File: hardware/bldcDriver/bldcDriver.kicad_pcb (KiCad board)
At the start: 2 copper layers, 89.8 x 41.5 mm, 4 parts

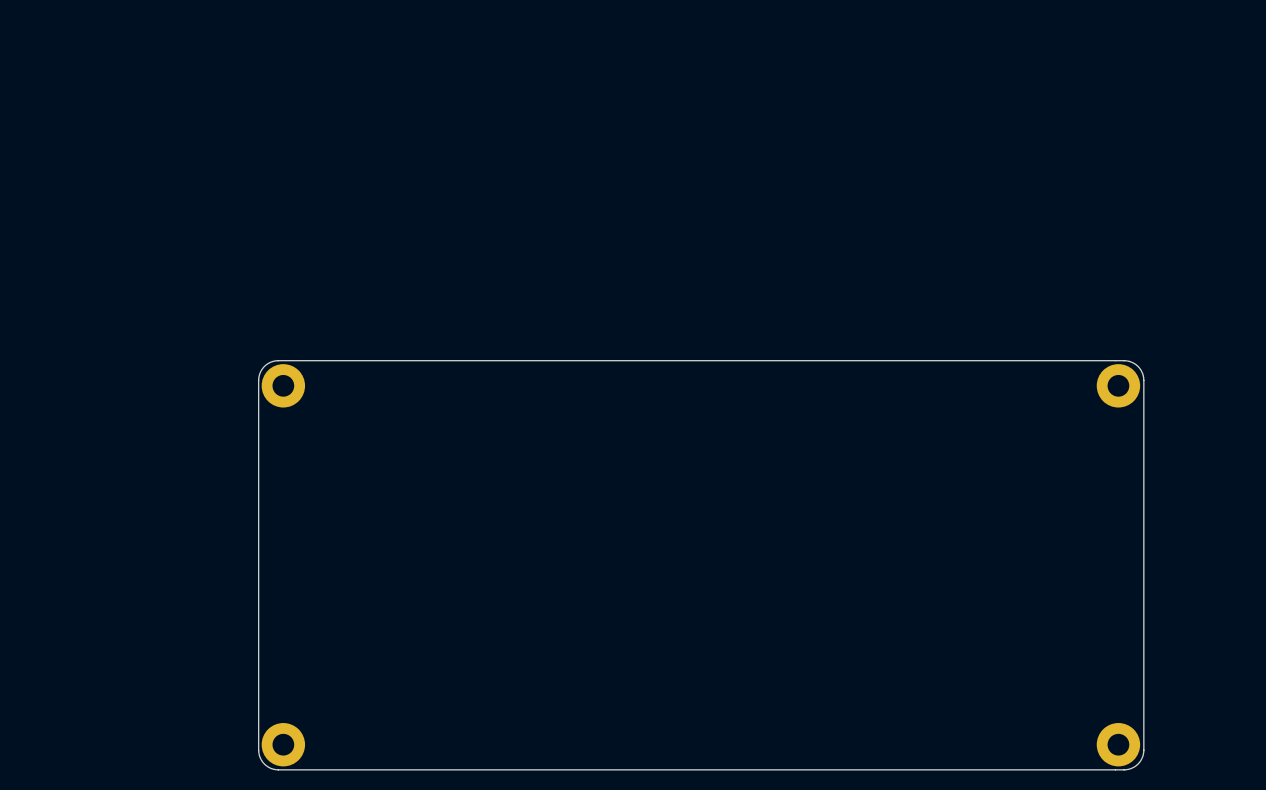
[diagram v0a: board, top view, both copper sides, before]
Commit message: update driver pcb
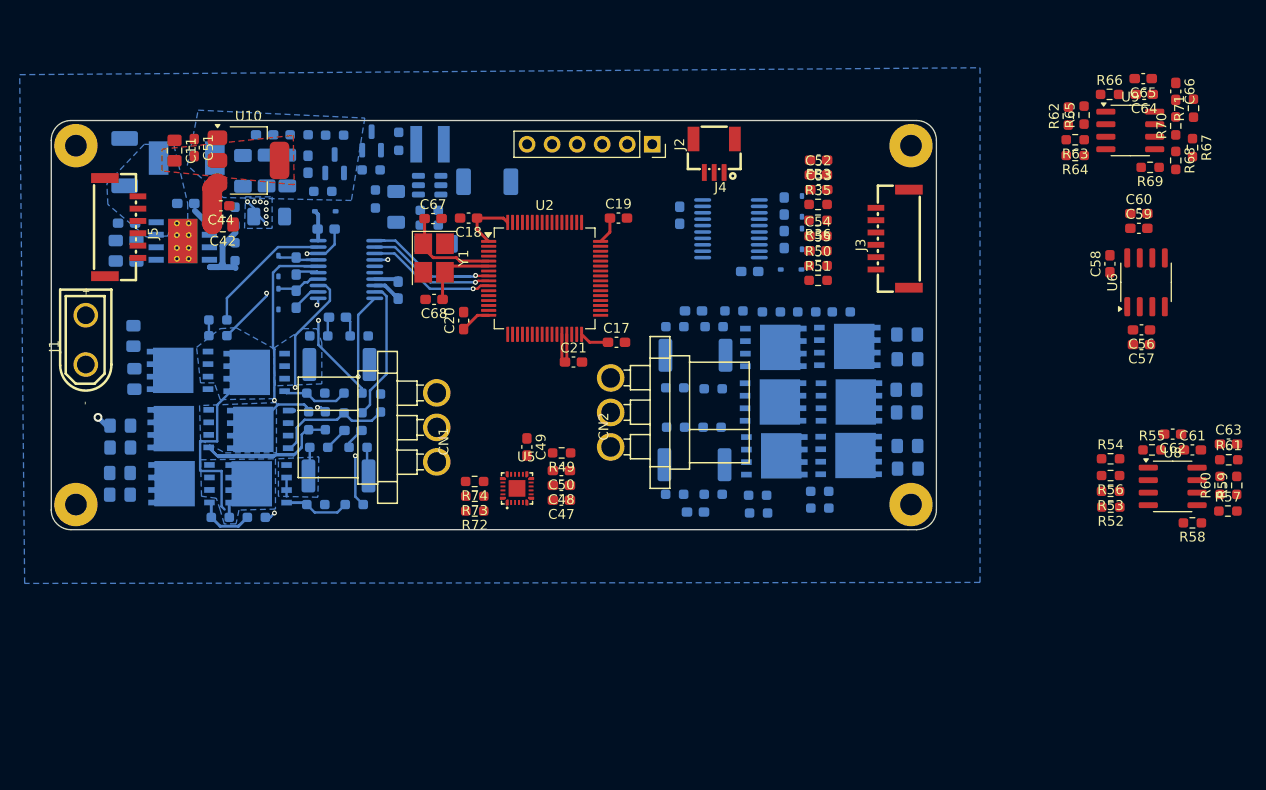
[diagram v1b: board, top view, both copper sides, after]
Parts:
- added C1: 10n, Capacitor_SMD:C_0603_1608Metric_Pad1.08x0.95mm_HandSolder, B.Cu at (46.1, 39.1)
- added C10: 47u, Capacitor_SMD:C_1206_3216Metric_Pad1.33x1.80mm_HandSolder, B.Cu at (71.5, 43.2)
- added C11: 10u, Capacitor_SMD:C_0805_2012Metric_Pad1.18x1.45mm_HandSolder, F.Cu at (45.0, 33.7)
- added C12: 100nF/25V, Capacitor_SMD:C_0603_1608Metric_Pad1.08x0.95mm_HandSolder, B.Cu at (96.2, 40.3)
- added C14: 100n, Capacitor_SMD:C_0603_1608Metric_Pad1.08x0.95mm_HandSolder, B.Cu at (103.3, 46.0)
- added C15: 100n, Capacitor_SMD:C_0603_1608Metric_Pad1.08x0.95mm_HandSolder, B.Cu at (106.8, 42.8)
- added C16: 100n, Capacitor_SMD:C_0603_1608Metric_Pad1.08x0.95mm_HandSolder, B.Cu at (106.8, 39.4)
- added C17: 100n, Capacitor_SMD:C_0603_1608Metric_Pad1.08x0.95mm_HandSolder, F.Cu at (89.8, 53.2)
- added C18: 100n, Capacitor_SMD:C_0603_1608Metric_Pad1.08x0.95mm_HandSolder, F.Cu at (74.8, 40.6)
- added C19: 100n, Capacitor_SMD:C_0603_1608Metric_Pad1.08x0.95mm_HandSolder, F.Cu at (90.0, 40.6)
- added C2: 47u, Capacitor_SMD:C_1206_3216Metric_Pad1.33x1.80mm_HandSolder, B.Cu at (56.4, 35.8)
- added C20: 100n, Capacitor_SMD:C_0603_1608Metric_Pad1.08x0.95mm_HandSolder, F.Cu at (74.3, 51.0)
- added C21: 470n, Capacitor_SMD:C_0603_1608Metric_Pad1.08x0.95mm_HandSolder, F.Cu at (85.4, 55.2)
- added C25: 100nF/25V, Capacitor_SMD:C_0603_1608Metric_Pad1.08x0.95mm_HandSolder, B.Cu at (67.6, 47.9)
- added C26: 100n, Capacitor_SMD:C_0603_1608Metric_Pad1.08x0.95mm_HandSolder, B.Cu at (60.3, 41.7)
- added C27: 100n, Capacitor_SMD:C_0603_1608Metric_Pad1.08x0.95mm_HandSolder, B.Cu at (57.3, 45.5)
- added C28: 100n, Capacitor_SMD:C_0603_1608Metric_Pad1.08x0.95mm_HandSolder, B.Cu at (57.3, 48.8)
- added C29: 22uF/25V, Capacitor_SMD:C_0805_2012Metric_Pad1.18x1.45mm_HandSolder, B.Cu at (40.8, 52.5)
- added C3: 47u, Capacitor_SMD:C_1206_3216Metric_Pad1.33x1.80mm_HandSolder, B.Cu at (54.3, 35.8)
- added C30: 1n, Capacitor_SMD:C_0603_1608Metric_Pad1.08x0.95mm_HandSolder, B.Cu at (61.5, 50.6)
- added C31: 22uF/25V, Capacitor_SMD:C_0805_2012Metric_Pad1.18x1.45mm_HandSolder, B.Cu at (119.3, 52.4)
- added C32: 1n, Capacitor_SMD:C_0603_1608Metric_Pad1.08x0.95mm_HandSolder, B.Cu at (97.6, 50.0)
- added C33: 22uF/25V, Capacitor_SMD:C_0805_2012Metric_Pad1.18x1.45mm_HandSolder, B.Cu at (40.9, 56.9)
- added C34: 22uF/25V, Capacitor_SMD:C_0805_2012Metric_Pad1.18x1.45mm_HandSolder, B.Cu at (119.3, 54.9)
- added C35: 22uF/25V, Capacitor_SMD:C_0805_2012Metric_Pad1.18x1.45mm_HandSolder, B.Cu at (39.4, 66.4)
- added C36: 1n, Capacitor_SMD:C_0603_1608Metric_Pad1.08x0.95mm_HandSolder, B.Cu at (63.1, 62.1)
- added C37: 22uF/25V, Capacitor_SMD:C_0805_2012Metric_Pad1.18x1.45mm_HandSolder, B.Cu at (119.3, 66.0)
- added C38: 1n, Capacitor_SMD:C_0603_1608Metric_Pad1.08x0.95mm_HandSolder, B.Cu at (97.8, 70.4)
- added C39: 22uF/25V, Capacitor_SMD:C_0805_2012Metric_Pad1.18x1.45mm_HandSolder, B.Cu at (39.4, 68.6)
- added C4: 47u, Capacitor_SMD:C_1206_3216Metric_Pad1.33x1.80mm_HandSolder, B.Cu at (51.9, 35.8)
- added C40: 22uF/25V, Capacitor_SMD:C_0805_2012Metric_Pad1.18x1.45mm_HandSolder, B.Cu at (119.3, 63.7)
- added C41: 22uF/25V, Capacitor_SMD:C_0805_2012Metric_Pad1.18x1.45mm_HandSolder, B.Cu at (39.5, 61.6)
- added C42: 10u, Capacitor_SMD:C_0805_2012Metric_Pad1.18x1.45mm_HandSolder, F.Cu at (49.9, 41.2)
- added C43: 22uF/25V, Capacitor_SMD:C_0805_2012Metric_Pad1.18x1.45mm_HandSolder, B.Cu at (119.2, 58.0)
- added C44: 100n, Capacitor_SMD:C_0603_1608Metric_Pad1.08x0.95mm_HandSolder, F.Cu at (49.7, 39.3)
- added C45: 22uF/25V, Capacitor_SMD:C_0805_2012Metric_Pad1.18x1.45mm_HandSolder, B.Cu at (39.5, 63.9)
- added C46: 22uF/25V, Capacitor_SMD:C_0805_2012Metric_Pad1.18x1.45mm_HandSolder, B.Cu at (119.2, 60.3)
- added C47: 10n, Capacitor_SMD:C_0603_1608Metric_Pad1.08x0.95mm_HandSolder, F.Cu at (84.2, 69.2)
- added C48: 100n, Capacitor_SMD:C_0603_1608Metric_Pad1.08x0.95mm_HandSolder, F.Cu at (84.2, 67.7)
- added C49: 2.2U, Capacitor_SMD:C_0603_1608Metric_Pad1.08x0.95mm_HandSolder, F.Cu at (80.7, 63.8)
- added C5: 22u, Capacitor_SMD:C_0805_2012Metric_Pad1.18x1.45mm_HandSolder, B.Cu at (39.0, 43.9)
- added C50: 100n, Capacitor_SMD:C_0603_1608Metric_Pad1.08x0.95mm_HandSolder, F.Cu at (84.2, 66.2)
- added C51: 100n, Capacitor_SMD:C_0603_1608Metric_Pad1.08x0.95mm_HandSolder, F.Cu at (47.0, 33.4)
- added C52: 4.7u, Capacitor_SMD:C_0603_1608Metric_Pad1.08x0.95mm_HandSolder, F.Cu at (110.3, 36.2)
- added C53: 100n, Capacitor_SMD:C_0603_1608Metric_Pad1.08x0.95mm_HandSolder, F.Cu at (110.3, 37.7)
- added C54: 4.7u, Capacitor_SMD:C_0603_1608Metric_Pad1.08x0.95mm_HandSolder, F.Cu at (110.2, 42.4)
- added C55: 100n, Capacitor_SMD:C_0603_1608Metric_Pad1.08x0.95mm_HandSolder, F.Cu at (110.2, 43.9)
- added C56: 4.7u, Capacitor_SMD:C_0603_1608Metric_Pad1.08x0.95mm_HandSolder, F.Cu at (143.0, 51.9)
- added C57: 100n, Capacitor_SMD:C_0603_1608Metric_Pad1.08x0.95mm_HandSolder, F.Cu at (143.0, 53.4)
- added C58: 100n, Capacitor_SMD:C_0603_1608Metric_Pad1.08x0.95mm_HandSolder, F.Cu at (139.8, 45.2)
- added C59: 4.7u, Capacitor_SMD:C_0603_1608Metric_Pad1.08x0.95mm_HandSolder, F.Cu at (142.8, 41.6)
- added C6: 22u, Capacitor_SMD:C_0805_2012Metric_Pad1.18x1.45mm_HandSolder, B.Cu at (41.1, 43.9)
- added C60: 100n, Capacitor_SMD:C_0603_1608Metric_Pad1.08x0.95mm_HandSolder, F.Cu at (142.8, 40.1)
- added C61: 100n, Capacitor_SMD:C_0603_1608Metric_Pad1.08x0.95mm_HandSolder, F.Cu at (148.2, 64.1)
- added C62: 2.2n, Capacitor_SMD:C_0603_1608Metric_Pad1.08x0.95mm_HandSolder, F.Cu at (146.2, 62.5)
- added C63: 2.2n, Capacitor_SMD:C_0603_1608Metric_Pad1.08x0.95mm_HandSolder, F.Cu at (151.9, 63.5)
- added C64: 2.2n, Capacitor_SMD:C_0603_1608Metric_Pad1.08x0.95mm_HandSolder, F.Cu at (143.3, 28.0)
- added C65: 2.2n, Capacitor_SMD:C_0603_1608Metric_Pad1.08x0.95mm_HandSolder, F.Cu at (143.2, 26.4)
- added C66: 100n, Capacitor_SMD:C_0603_1608Metric_Pad1.08x0.95mm_HandSolder, F.Cu at (146.5, 27.7)
- added C67: 12p, Capacitor_SMD:C_0603_1608Metric_Pad1.08x0.95mm_HandSolder, F.Cu at (71.2, 40.6)
- added C68: 12p, Capacitor_SMD:C_0603_1608Metric_Pad1.08x0.95mm_HandSolder, F.Cu at (71.3, 48.8)
- added C7: 100n, Capacitor_SMD:C_0603_1608Metric_Pad1.08x0.95mm_HandSolder, B.Cu at (40.1, 41.1)
- added C8: 100n, Capacitor_SMD:C_0603_1608Metric_Pad1.08x0.95mm_HandSolder, B.Cu at (58.5, 35.1)
- added C9: 47u, Capacitor_SMD:C_1206_3216Metric_Pad1.33x1.80mm_HandSolder, B.Cu at (67.4, 39.5)
- added CN1: MR30PW-F, balancerDriver:CONN-TH_MR30PW-F, F.Cu at (69.1, 61.8)
- added CN2: MR30PW-F, balancerDriver:CONN-TH_MR30PW-F, F.Cu at (91.7, 60.3)
- added D1: LED, LED_SMD:LED_0603_1608Metric_Pad1.05x0.95mm_HandSolder, B.Cu at (54.1, 32.1)
- added D10: 1N5819WS, Diode_SMD:D_SOD-323, B.Cu at (60.2, 39.9)
- added D11: 1N5819WS, Diode_SMD:D_SOD-323, B.Cu at (55.5, 45.5)
- added D12: 1N5819WS, Diode_SMD:D_SOD-323, B.Cu at (55.5, 48.8)
- added D2: 1N5819WS, Diode_SMD:D_SOD-323, B.Cu at (107.5, 45.8)
- added D3: 1N5819WS, Diode_SMD:D_SOD-323, B.Cu at (108.6, 42.7)
- added D4: 1N5819WS, Diode_SMD:D_SOD-323, B.Cu at (108.6, 39.4)
- added D8: 1N5712UR, Diode_SMD:D_MELF, B.Cu at (39.9, 34.9)
- added D9: 1N5712UR, Diode_SMD:D_MELF, B.Cu at (76.7, 36.9)
- added FB2: FerriteBead, Capacitor_SMD:C_1206_3216Metric_Pad1.33x1.80mm_HandSolder, B.Cu at (54.6, 40.4)
- added FB3: FerriteBead, Capacitor_SMD:C_0603_1608Metric_Pad1.08x0.95mm_HandSolder, F.Cu at (110.3, 34.7)
- added J1: Conn_01x02, balancerDriver:CONN-TH_XT30UPB-M, F.Cu at (36.0, 52.9)
- added J2: Conn_01x06, Connector_PinSocket_2.54mm:PinSocket_1x06_P2.54mm_Vertical, F.Cu at (93.4, 33.1)
- added J3: Conn_01x06, balancerDriver:CONN-SMD_BM06B-GHS-TBT-LF-SN, F.Cu at (117.8, 42.7)
- added J4: Conn_01x03, balancerDriver:CONN-SMD_3P-P1.00_WAFER-SH1.0-3PWB, F.Cu at (99.7, 34.3)
- added J5: Conn_01x06, balancerDriver:CONN-SMD_BM06B-GHS-TBT-LF-SN, F.Cu at (39.6, 41.5)
- added L1: 10u, Inductor_SMD:L_Sumida_CDMC6D28_7.25x6.5mm, B.Cu at (46.2, 34.5)
- added L2: 10u, Inductor_SMD:L_Taiyo-Yuden_MD-4040, B.Cu at (70.9, 33.1)
- added Q1: KNY3406C, balancerDriver:PDFN-8_L4.9-W5.8-P1.27-LS6.1-BL, B.Cu at (45.5, 56.0)
- added Q10: KNY3406C, balancerDriver:PDFN-8_L4.9-W5.8-P1.27-LS6.1-BL, B.Cu at (53.7, 62.0)
- added Q11: KNY3406C, balancerDriver:PDFN-8_L4.9-W5.8-P1.27-LS6.1-BL, B.Cu at (113.4, 59.2)
- added Q12: KNY3406C, balancerDriver:PDFN-8_L4.9-W5.8-P1.27-LS6.1-BL, B.Cu at (105.7, 59.2)
- added Q13: PMOS, Package_TO_SOT_SMD:SOT-23, B.Cu at (61.2, 35.1)
- added Q14: S8050, Package_TO_SOT_SMD:SOT-23, B.Cu at (65.0, 32.8)
- added Q2: KNY3406C, balancerDriver:PDFN-8_L4.9-W5.8-P1.27-LS6.1-BL, B.Cu at (53.3, 56.2)
- added Q3: KNY3406C, balancerDriver:PDFN-8_L4.9-W5.8-P1.27-LS6.1-BL, B.Cu at (113.2, 53.6)
- added Q4: KNY3406C, balancerDriver:PDFN-8_L4.9-W5.8-P1.27-LS6.1-BL, B.Cu at (105.7, 53.7)
- added Q5: KNY3406C, balancerDriver:PDFN-8_L4.9-W5.8-P1.27-LS6.1-BL, B.Cu at (45.7, 67.5)
- added Q6: KNY3406C, balancerDriver:PDFN-8_L4.9-W5.8-P1.27-LS6.1-BL, B.Cu at (53.5, 67.5)
- added Q7: KNY3406C, balancerDriver:PDFN-8_L4.9-W5.8-P1.27-LS6.1-BL, B.Cu at (113.3, 64.7)
- added Q8: KNY3406C, balancerDriver:PDFN-8_L4.9-W5.8-P1.27-LS6.1-BL, B.Cu at (105.8, 64.7)
- added Q9: KNY3406C, balancerDriver:PDFN-8_L4.9-W5.8-P1.27-LS6.1-BL, B.Cu at (45.6, 61.9)
- added R1: 10k, Resistor_SMD:R_0603_1608Metric_Pad0.98x0.95mm_HandSolder, B.Cu at (51.1, 40.4)
- added R10: 100R, Resistor_SMD:R_0603_1608Metric_Pad0.98x0.95mm_HandSolder, B.Cu at (95.7, 51.6)
- added R11: 20mR, Resistor_SMD:R_2512_6332Metric_Pad1.40x3.35mm_HandSolder, B.Cu at (61.7, 55.4)
- added R12: 20mR, Resistor_SMD:R_2512_6332Metric_Pad1.40x3.35mm_HandSolder, B.Cu at (97.8, 54.5)
- added R13: 10k, Resistor_SMD:R_0603_1608Metric_Pad0.98x0.95mm_HandSolder, B.Cu at (49.4, 52.5)
- added R14: 10k, Resistor_SMD:R_0603_1608Metric_Pad0.98x0.95mm_HandSolder, B.Cu at (59.3, 58.3)
- added R15: 10k, Resistor_SMD:R_0603_1608Metric_Pad0.98x0.95mm_HandSolder, B.Cu at (112.6, 50.1)
- added R16: 10k, Resistor_SMD:R_0603_1608Metric_Pad0.98x0.95mm_HandSolder, B.Cu at (105.5, 50.1)
- added R17: 10R, Resistor_SMD:R_0603_1608Metric_Pad0.98x0.95mm_HandSolder, B.Cu at (49.4, 50.9)
- added R18: 10R, Resistor_SMD:R_0603_1608Metric_Pad0.98x0.95mm_HandSolder, B.Cu at (63.1, 58.3)
- added R19: 10R, Resistor_SMD:R_0603_1608Metric_Pad0.98x0.95mm_HandSolder, B.Cu at (109.1, 50.1)
- added R2: 3.3k, Resistor_SMD:R_0603_1608Metric_Pad0.98x0.95mm_HandSolder, B.Cu at (51.1, 44.0)
- added R20: 10R, Resistor_SMD:R_0603_1608Metric_Pad0.98x0.95mm_HandSolder, B.Cu at (101.7, 50.0)
- added R21: 100R, Resistor_SMD:R_0603_1608Metric_Pad0.98x0.95mm_HandSolder, B.Cu at (59.6, 63.8)
- added R22: 100R, Resistor_SMD:R_0603_1608Metric_Pad0.98x0.95mm_HandSolder, B.Cu at (63.6, 63.8)
- added R23: 100R, Resistor_SMD:R_0603_1608Metric_Pad0.98x0.95mm_HandSolder, B.Cu at (99.6, 68.6)
- added R24: 100R, Resistor_SMD:R_0603_1608Metric_Pad0.98x0.95mm_HandSolder, B.Cu at (95.7, 68.6)
- added R25: 20mR, Resistor_SMD:R_2512_6332Metric_Pad1.40x3.35mm_HandSolder, B.Cu at (61.6, 66.7)
- added R26: 20mR, Resistor_SMD:R_2512_6332Metric_Pad1.40x3.35mm_HandSolder, B.Cu at (97.7, 65.6)
- added R27: 10k, Resistor_SMD:R_0603_1608Metric_Pad0.98x0.95mm_HandSolder, B.Cu at (49.6, 70.9)
- added R28: 10k, Resistor_SMD:R_0603_1608Metric_Pad0.98x0.95mm_HandSolder, B.Cu at (59.3, 69.6)
- added R29: 10k, Resistor_SMD:R_0603_1608Metric_Pad0.98x0.95mm_HandSolder, B.Cu at (110.4, 68.3)
- added R3: 4.7k, Resistor_SMD:R_0603_1608Metric_Pad0.98x0.95mm_HandSolder, B.Cu at (57.6, 32.1)
- added R30: 10k, Resistor_SMD:R_0603_1608Metric_Pad0.98x0.95mm_HandSolder, B.Cu at (104.1, 68.7)
- added R31: 10R, Resistor_SMD:R_0603_1608Metric_Pad0.98x0.95mm_HandSolder, B.Cu at (53.3, 70.9)
- added R32: 10R, Resistor_SMD:R_0603_1608Metric_Pad0.98x0.95mm_HandSolder, B.Cu at (63.2, 69.6)
- added R33: 10R, Resistor_SMD:R_0603_1608Metric_Pad0.98x0.95mm_HandSolder, B.Cu at (110.4, 70.0)
- added R34: 10R, Resistor_SMD:R_0603_1608Metric_Pad0.98x0.95mm_HandSolder, B.Cu at (104.2, 70.5)
- added R35: 1k, Resistor_SMD:R_0603_1608Metric_Pad0.98x0.95mm_HandSolder, F.Cu at (110.2, 39.2)
- added R36: 1k, Resistor_SMD:R_0603_1608Metric_Pad0.98x0.95mm_HandSolder, F.Cu at (110.2, 40.8)
- added R37: 10k, Resistor_SMD:R_0603_1608Metric_Pad0.98x0.95mm_HandSolder, B.Cu at (64.9, 35.7)
- added R38: 10k, Resistor_SMD:R_0603_1608Metric_Pad0.98x0.95mm_HandSolder, B.Cu at (65.3, 38.6)
- added R39: 63.4k, Resistor_SMD:R_0603_1608Metric_Pad0.98x0.95mm_HandSolder, B.Cu at (70.8, 41.3)
- added R4: 10k, Resistor_SMD:R_0603_1608Metric_Pad0.98x0.95mm_HandSolder, B.Cu at (60.0, 37.9)
- added R40: 3.3k, Resistor_SMD:R_0603_1608Metric_Pad0.98x0.95mm_HandSolder, B.Cu at (70.8, 39.8)
- added R41: 10k, Resistor_SMD:R_0603_1608Metric_Pad0.98x0.95mm_HandSolder, B.Cu at (58.6, 61.1)
- added R42: 10k, Resistor_SMD:R_0603_1608Metric_Pad0.98x0.95mm_HandSolder, B.Cu at (65.9, 59.3)
- added R43: 10k, Resistor_SMD:R_0603_1608Metric_Pad0.98x0.95mm_HandSolder, B.Cu at (99.5, 61.8)
- added R44: 10k, Resistor_SMD:R_0603_1608Metric_Pad0.98x0.95mm_HandSolder, B.Cu at (99.6, 57.9)
- added R45: 10R, Resistor_SMD:R_0603_1608Metric_Pad0.98x0.95mm_HandSolder, B.Cu at (60.3, 61.1)
- added R46: 10R, Resistor_SMD:R_0603_1608Metric_Pad0.98x0.95mm_HandSolder, B.Cu at (63.1, 60.3)
- added R47: 10R, Resistor_SMD:R_0603_1608Metric_Pad0.98x0.95mm_HandSolder, B.Cu at (95.8, 61.8)
- added R48: 10R, Resistor_SMD:R_0603_1608Metric_Pad0.98x0.95mm_HandSolder, B.Cu at (95.7, 57.8)
- added R49: 10K, Resistor_SMD:R_0603_1608Metric_Pad0.98x0.95mm_HandSolder, F.Cu at (84.2, 64.4)
- added R5: 100R, Resistor_SMD:R_0603_1608Metric_Pad0.98x0.95mm_HandSolder, B.Cu at (61.2, 32.2)
- added R50: 1k, Resistor_SMD:R_0603_1608Metric_Pad0.98x0.95mm_HandSolder, F.Cu at (110.2, 45.4)
- added R51: 1k, Resistor_SMD:R_0603_1608Metric_Pad0.98x0.95mm_HandSolder, F.Cu at (110.2, 46.9)
- added R52: 10k, Resistor_SMD:R_0603_1608Metric_Pad0.98x0.95mm_HandSolder, F.Cu at (139.9, 69.9)
- added R53: 1k, Resistor_SMD:R_0603_1608Metric_Pad0.98x0.95mm_HandSolder, F.Cu at (139.9, 68.3)
- added R54: 10k, Resistor_SMD:R_0603_1608Metric_Pad0.98x0.95mm_HandSolder, F.Cu at (139.9, 65.0)
- added R55: 100R, Resistor_SMD:R_0603_1608Metric_Pad0.98x0.95mm_HandSolder, F.Cu at (144.1, 64.1)
- added R56: 1k, Resistor_SMD:R_0603_1608Metric_Pad0.98x0.95mm_HandSolder, F.Cu at (139.9, 66.7)
- added R57: 1k, Resistor_SMD:R_0603_1608Metric_Pad0.98x0.95mm_HandSolder, F.Cu at (151.8, 70.3)
- added R58: 10k, Resistor_SMD:R_0603_1608Metric_Pad0.98x0.95mm_HandSolder, F.Cu at (148.2, 71.5)
- added R59: 1k, Resistor_SMD:R_0603_1608Metric_Pad0.98x0.95mm_HandSolder, F.Cu at (152.7, 67.7)
- added R6: 1k, Resistor_SMD:R_0603_1608Metric_Pad0.98x0.95mm_HandSolder, B.Cu at (67.7, 32.8)
- added R60: 10k, Resistor_SMD:R_0603_1608Metric_Pad0.98x0.95mm_HandSolder, F.Cu at (151.0, 67.7)
- added R61: 100R, Resistor_SMD:R_0603_1608Metric_Pad0.98x0.95mm_HandSolder, F.Cu at (151.9, 65.1)
- added R62: 1k, Resistor_SMD:R_0603_1608Metric_Pad0.98x0.95mm_HandSolder, F.Cu at (135.6, 30.2)
- added R63: 1k, Resistor_SMD:R_0603_1608Metric_Pad0.98x0.95mm_HandSolder, F.Cu at (136.3, 32.6)
- added R64: 10k, Resistor_SMD:R_0603_1608Metric_Pad0.98x0.95mm_HandSolder, F.Cu at (136.3, 34.2)
- added R65: 10k, Resistor_SMD:R_0603_1608Metric_Pad0.98x0.95mm_HandSolder, F.Cu at (137.2, 30.1)
- added R66: 100R, Resistor_SMD:R_0603_1608Metric_Pad0.98x0.95mm_HandSolder, F.Cu at (139.8, 28.0)
- added R67: 1k, Resistor_SMD:R_0603_1608Metric_Pad0.98x0.95mm_HandSolder, F.Cu at (148.2, 33.4)
- added R68: 1k, Resistor_SMD:R_0603_1608Metric_Pad0.98x0.95mm_HandSolder, F.Cu at (146.5, 34.7)
- added R69: 10k, Resistor_SMD:R_0603_1608Metric_Pad0.98x0.95mm_HandSolder, F.Cu at (143.9, 35.4)
- added R7: 100R, Resistor_SMD:R_0603_1608Metric_Pad0.98x0.95mm_HandSolder, B.Cu at (59.6, 52.5)
- added R70: 10k, Resistor_SMD:R_0603_1608Metric_Pad0.98x0.95mm_HandSolder, F.Cu at (146.5, 31.2)
- added R71: 100R, Resistor_SMD:R_0603_1608Metric_Pad0.98x0.95mm_HandSolder, F.Cu at (148.3, 29.4)
- added R72: 4.7k, Resistor_SMD:R_0603_1608Metric_Pad0.98x0.95mm_HandSolder, F.Cu at (75.4, 70.3)
- added R73: 4.7k, Resistor_SMD:R_0603_1608Metric_Pad0.98x0.95mm_HandSolder, F.Cu at (75.4, 68.8)
- added R74: 4.7k, Resistor_SMD:R_0603_1608Metric_Pad0.98x0.95mm_HandSolder, F.Cu at (75.4, 67.3)
- added R8: 100R, Resistor_SMD:R_0603_1608Metric_Pad0.98x0.95mm_HandSolder, B.Cu at (63.7, 52.5)
- added R9: 100R, Resistor_SMD:R_0603_1608Metric_Pad0.98x0.95mm_HandSolder, B.Cu at (99.7, 51.6)
- added U1: FD6288T, balancerDriver:TSSOP-20_L6.5-W4.4-P0.65-LS6.4-BL, B.Cu at (101.4, 41.7)
- added U10: AMS1117, Package_TO_SOT_SMD:SOT-223-3_TabPin2, F.Cu at (52.5, 34.7)
- added U11: FD6288T, balancerDriver:TSSOP-20_L6.5-W4.4-P0.65-LS6.4-BL, B.Cu at (62.4, 45.8)
- added U2: STM32G431RBTx, Package_QFP:LQFP-64_10x10mm_P0.5mm, F.Cu at (82.5, 46.7)
- added U3: TPS5430DDA, Package_SO:TI_SO-PowerPAD-8_ThermalVias, B.Cu at (45.8, 42.9)
- added U5: MPU6500, balancerDriver:QFN-24_L3.0-W3.0-P0.40-BL-EP, F.Cu at (79.7, 68.0)
- added U6: TLV9062xD, Package_SO:SOIC-8_3.9x4.9mm_P1.27mm, F.Cu at (143.5, 47.1)
- added U7: MT3608, Package_TO_SOT_SMD:SOT-23-6, B.Cu at (70.8, 37.2)
- added U8: TLV9062xD, Package_SO:SOIC-8_3.9x4.9mm_P1.27mm, F.Cu at (146.2, 67.8)
- added U9: TLV9062xD, Package_SO:SOIC-8_3.9x4.9mm_P1.27mm, F.Cu at (141.9, 31.7)
- added Y1: 25MHz, Crystal:Crystal_SMD_SeikoEpson_FA238-4Pin_3.2x2.5mm_HandSoldering, F.Cu at (71.3, 44.6)
- moved ? 32.2 mm to (35.0, 33.2)
- moved ? 32.2 mm to (35.0, 69.6)
- moved ? 32.2 mm to (119.7, 33.2)
- moved ? 32.2 mm to (119.7, 69.6)
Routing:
- net /inverter/1SH_U: track 0.00 -> 35.7 mm, vias 0 -> 2
- net /inverter/1GH_B: track 0.00 -> 31.8 mm, vias 0 -> 2
- net Net-(Q9-G): track 0.00 -> 24.0 mm
- net /inverter/1GL_B: track 0.00 -> 22.1 mm, vias 0 -> 2
- net +3V3: track 0.00 -> 20.8 mm
- net /inverter/1GH_C: track 0.00 -> 16.8 mm, vias 0 -> 2
- net /TIM1_CH1: track 0.00 -> 16.5 mm, vias 0 -> 1
- net /inverter/1GL_C: track 0.00 -> 14.2 mm
- net /inverter/1GH_A: track 0.00 -> 13.6 mm
- net /TIM1_CH3: track 0.00 -> 13.2 mm, vias 0 -> 1
- net /TIM1_CH2: track 0.00 -> 13.1 mm, vias 0 -> 1
- net Net-(Q10-G): track 0.00 -> 12.4 mm
- net /inverter/1GL_A: track 0.00 -> 11.6 mm, vias 0 -> 2
- net /YI: track 0.00 -> 10.2 mm
- net /inverter/1SH_V: track 0.00 -> 9.31 mm
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- added copper zone on F.Cu, net +3V3
- added copper zone on B.Cu, net +5V
- added copper zone on B.Cu, net +BATT
- added copper zone on B.Cu, net /inverter/1SH_U
- added copper zone on B.Cu, net /inverter/1SH_V
- added copper zone on B.Cu, net /inverter/1SH_W
- added copper zone on B.Cu, net GNDD
- added copper zone on In2.Cu, net GNDPWR
- added copper zone on B.Cu, net Net-(D8-K)
- added copper zone on B.Cu, net Net-(Q2-S-Pad1)
- added copper zone on B.Cu, net Net-(Q6-S-Pad1)
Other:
- copper layers 2 -> 4

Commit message: update pcbs
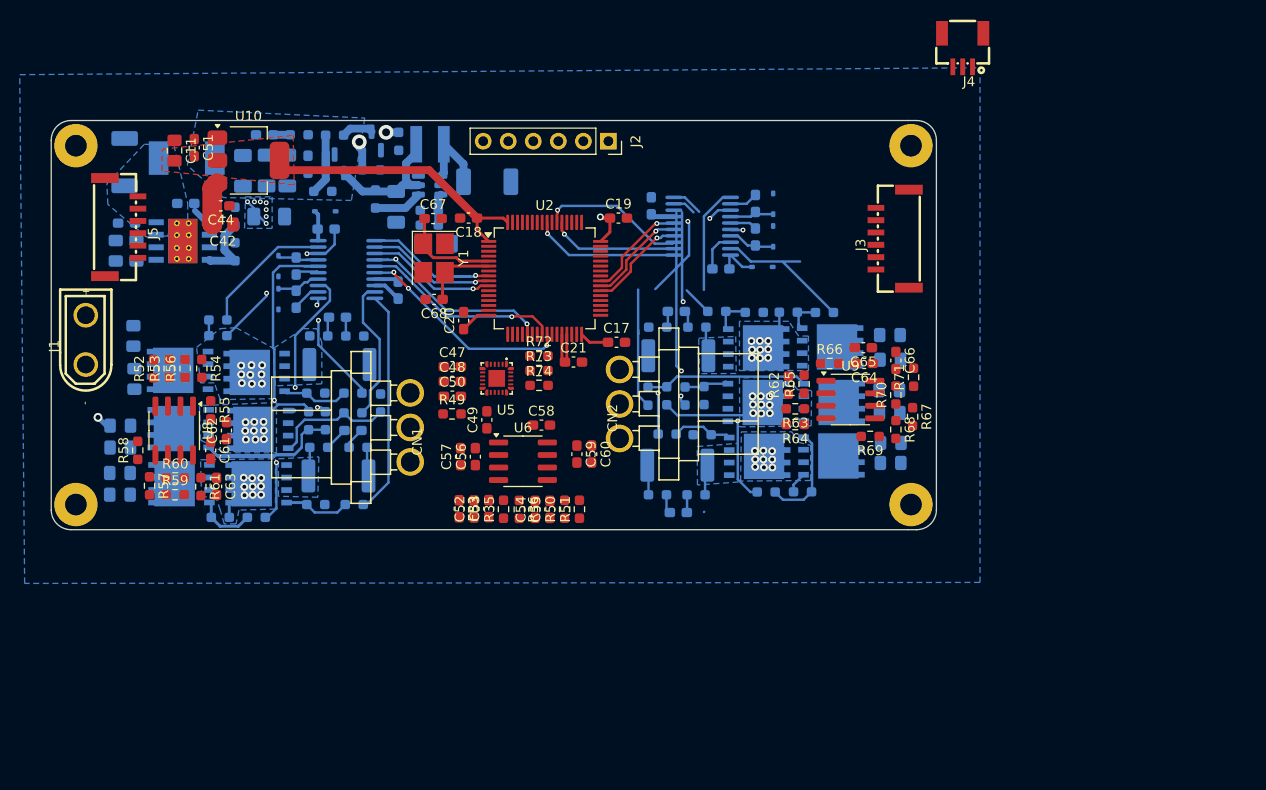
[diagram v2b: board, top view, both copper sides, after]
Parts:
- moved R57 109.4 mm to (42.4, 67.7), turned to -90 degrees
- moved R59 107.7 mm to (45.0, 68.6), turned to 0 degrees
- moved R58 107.2 mm to (41.2, 64.1), turned to 90 degrees
- moved R60 106.0 mm to (45.0, 66.9), turned to 0 degrees
- moved R61 104.3 mm to (47.6, 67.8), turned to -90 degrees
- moved C63 102.7 mm to (49.2, 67.8), turned to -90 degrees
- moved U8 101.4 mm to (44.9, 62.1), turned to -90 degrees
- moved C61 99.6 mm to (48.6, 64.1), turned to -90 degrees
- moved R52 98.1 mm to (42.8, 55.9), turned to 90 degrees
- moved R53 96.3 mm to (44.4, 55.8), turned to 90 degrees
- moved C62 96.0 mm to (50.2, 62.1), turned to 90 degrees
- moved R55 95.6 mm to (48.6, 60.0), turned to -90 degrees
- moved R56 94.5 mm to (46.0, 55.8), turned to 90 degrees
- moved R54 92.6 mm to (47.7, 55.8), turned to -90 degrees
- moved C57 70.0 mm to (74.0, 64.8), turned to 90 degrees
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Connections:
- C30 pad 1: /1A_iSENSOR_N -> /1A_ISENSOR_N
- C32 pad 1: /2A_iSENSOR_N -> /2A_ISENSOR_N
- C32 pad 2: /2A_iSENSOR_P -> /2A_ISENSOR_P
- C36 pad 1: /1B_iSENSOR_N -> /1B_ISENSOR_N
- C36 pad 2: /1B_iSENSOR_P -> /1B_ISENSOR_P
- C38 pad 1: /2B_iSENSOR_N -> /2B_ISENSOR_N
- C38 pad 2: /2B_iSENSOR_P -> /2B_ISENSOR_P
- CN2 pad 1: /inverter/2SH_U -> /inverter/2SH_W
- CN2 pad 3: /inverter/2SH_W -> /inverter/2SH_U
- R10 pad 2: /2A_iSENSOR_N -> /2A_ISENSOR_N
- R21 pad 2: /1B_iSENSOR_P -> /1B_ISENSOR_P
- R22 pad 2: /1B_iSENSOR_N -> /1B_ISENSOR_N
- R23 pad 2: /2B_iSENSOR_P -> /2B_ISENSOR_P
- R24 pad 2: /2B_iSENSOR_N -> /2B_ISENSOR_N
- R8 pad 2: /1A_iSENSOR_N -> /1A_ISENSOR_N
- R9 pad 2: /2A_iSENSOR_P -> /2A_ISENSOR_P
- U2 pad 21: /TIM8_CH1N -> /TIM1_CH1N
- U2 pad 35: /TIM1_CH1N -> unconnected-(U2-PB13-Pad35)
- U2 pad 56: unconnected-(U2-PB3-Pad56) -> /TIM8_CH1N
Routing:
- net /inverter/2GH_B: track 0.00 -> 29.5 mm, vias 0 -> 2
- net /inverter/2SH_V: track 0.00 -> 28.0 mm, vias 0 -> 9
- net /inverter/2GL_B: track 0.00 -> 27.8 mm, vias 0 -> 2
- net /inverter/2GH_C: track 0.00 -> 26.4 mm, vias 0 -> 2
- net /inverter/2SH_U: track 0.00 -> 24.7 mm, vias 0 -> 9
- net +3V3: track 20.8 -> 44.5 mm, vias 0 -> 1
- net /inverter/2GL_C: track 0.00 -> 22.2 mm, vias 0 -> 2
- net /TIM1_CH3N: track 0.00 -> 22.1 mm, vias 0 -> 3
- net /inverter/2SH_W: track 0.00 -> 20.5 mm, vias 0 -> 9
- net /TIM1_CH2N: track 0.00 -> 20.4 mm, vias 0 -> 1
- net /inverter/1SH_W: track 4.72 -> 21.7 mm, vias 0 -> 9
- net /inverter/1SH_V: track 9.31 -> 26.1 mm, vias 0 -> 9
- net Net-(Q11-G): track 0.00 -> 16.6 mm
- net /TIM8_CH3N: track 0.00 -> 14.9 mm, vias 0 -> 1
- net /TIM8_CH1N: track 0.00 -> 14.9 mm, vias 0 -> 1
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- added copper zone on B.Cu, net /inverter/2SH_U
- added copper zone on B.Cu, net /inverter/2SH_V
- added copper zone on B.Cu, net /inverter/2SH_W
- added copper zone on B.Cu, net Net-(Q4-S-Pad1)
- added copper zone on B.Cu, net Net-(Q8-S-Pad1)

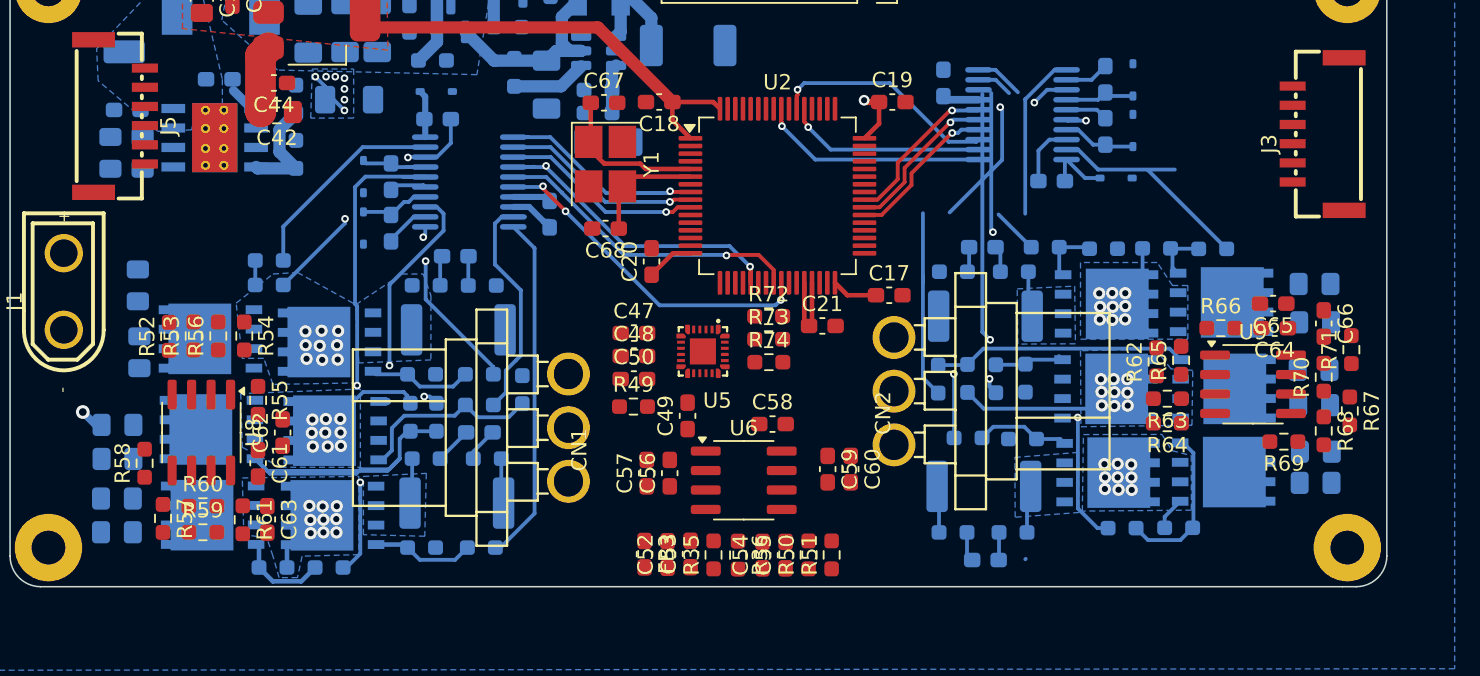
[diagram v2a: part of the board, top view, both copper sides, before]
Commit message: update pcbs
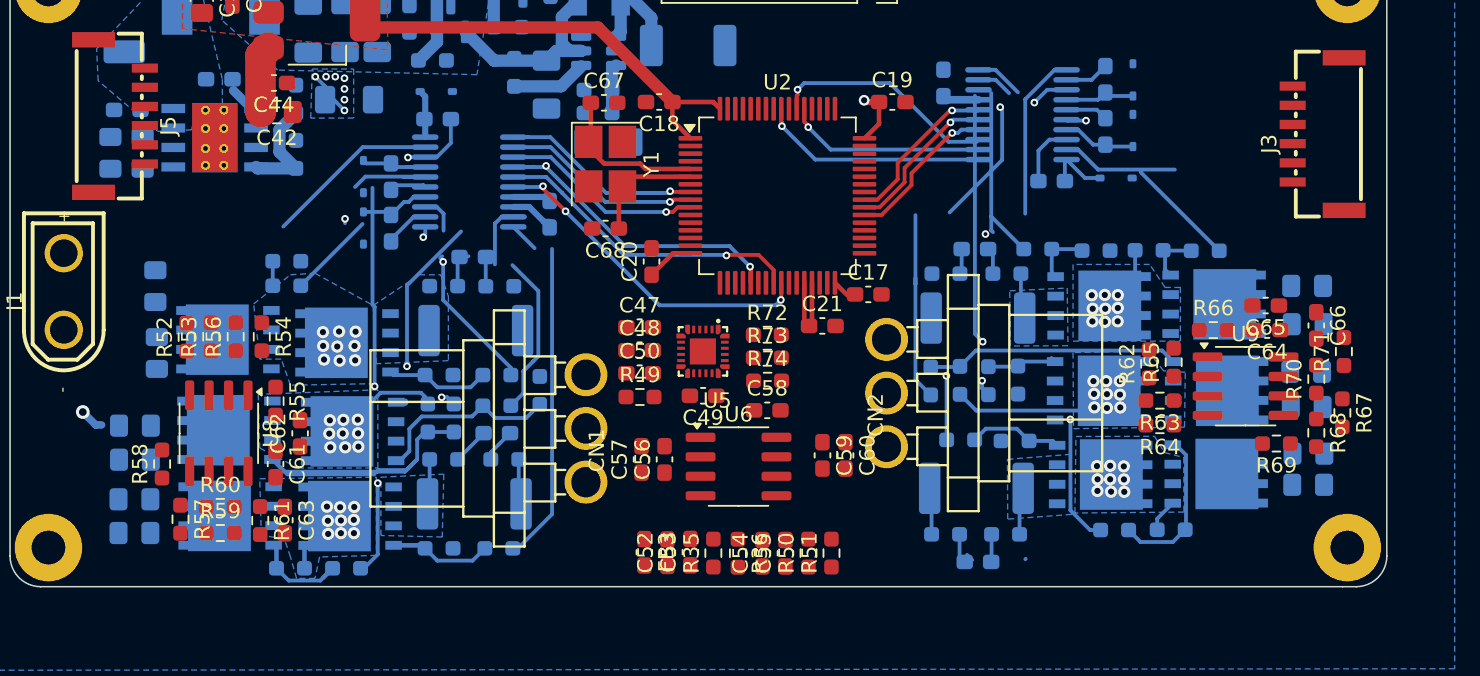
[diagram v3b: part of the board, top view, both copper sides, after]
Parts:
- moved C49 1.66 mm to (77.7, 59.7), turned to 180 degrees
- moved C17 1.37 mm to (88.4, 53.1)
- moved R72 1.21 mm to (81.8, 55.8)
- moved R73 1.21 mm to (81.8, 57.3)
- moved R74 1.21 mm to (81.9, 58.8)
- moved C63 1.14 mm to (50.4, 67.9)
- moved Q5 1.14 mm to (46.8, 67.6)
- moved R57 1.14 mm to (43.6, 67.8)
- moved C29 1.14 mm to (41.9, 52.6)
- moved C36 1.14 mm to (64.2, 62.2)
- moved R11 1.14 mm to (62.8, 55.5)
- moved R17 1.14 mm to (50.5, 51.0)
- moved R55 1.14 mm to (49.8, 60.1)
- moved R8 1.14 mm to (64.4, 52.6)
- moved C30 1.14 mm to (62.6, 50.7)
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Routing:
- net /inverter/1GH_A: track 13.6 -> 11.4 mm
- net +3V3: track 44.5 -> 42.6 mm
